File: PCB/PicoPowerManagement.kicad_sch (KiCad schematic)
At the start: 25 parts, among them J1 Conn_02x07_Odd_Even, J10 Conn_02x07_Odd_Even, J11 NAS Fan 1, J12 NAS Fan 2, J13 ATX 24P Connection, J15 Conn_01x02, J2 Conn_02x07_Odd_Even, J3 UART Header, J4 DEBUG, J5 SwitchLEDS, J6 Conn_02x07_Odd_Even, J7 Conn_02x07_Odd_Even, J8 PowerSwitch, J9 Conn_02x07_Odd_Even, Q1 2N3904, SW1 SW_SPST, U2 LP5810ADSDR, U3 LP5810ADSDR, U4 LSF0101DRYR, U5 LSF0101DRYR

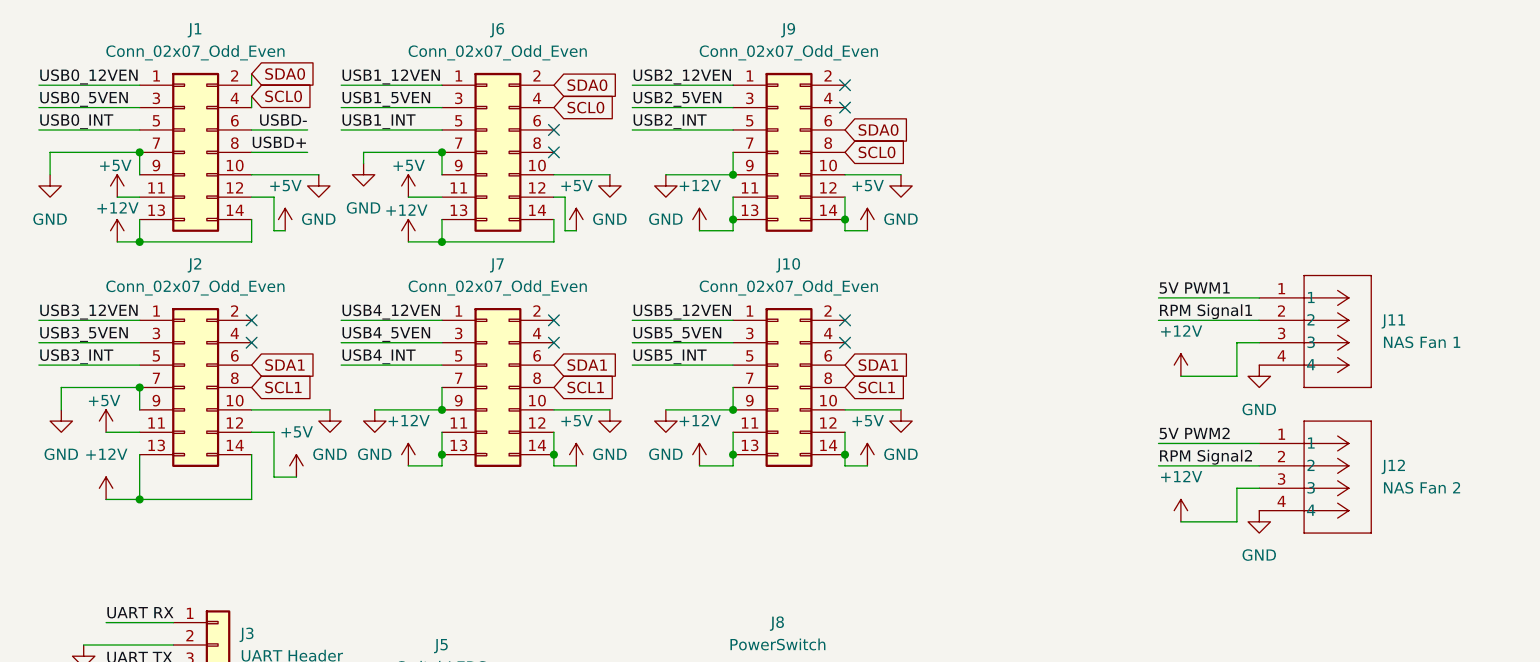
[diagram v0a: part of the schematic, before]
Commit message: confused now
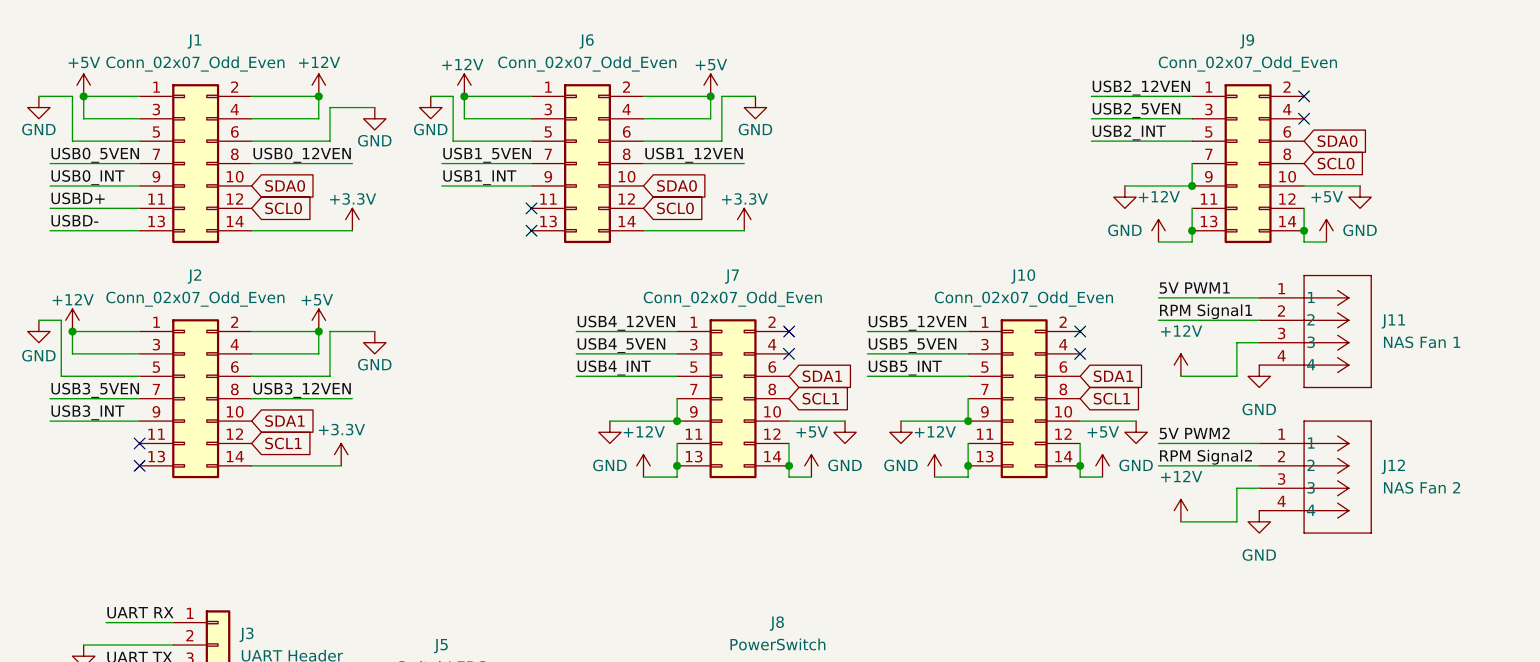
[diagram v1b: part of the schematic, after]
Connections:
- net +12V: now also J1.2 (Pin_2), J1.4 (Pin_4), J2.1 (Pin_1), J2.3 (Pin_3), J6.1 (Pin_1), J6.3 (Pin_3); no longer J1.13 (Pin_13), J1.14 (Pin_14), J2.13 (Pin_13), J2.14 (Pin_14), J6.13 (Pin_13), J6.14 (Pin_14)
- net +3.3V: now also J1.14 (Pin_14), J2.14 (Pin_14), J6.14 (Pin_14)
- net +5V: now also J1.1 (Pin_1), J1.3 (Pin_3), J2.2 (Pin_2), J2.4 (Pin_4), J6.2 (Pin_2), J6.4 (Pin_4); no longer J1.11 (Pin_11), J1.12 (Pin_12), J2.11 (Pin_11), J2.12 (Pin_12), J6.11 (Pin_11), J6.12 (Pin_12)
- net GND: now also J1.5 (Pin_5), J1.6 (Pin_6), J2.5 (Pin_5), J2.6 (Pin_6), J6.5 (Pin_5), J6.6 (Pin_6); no longer J1.10 (Pin_10), J1.7 (Pin_7), J1.9 (Pin_9), J2.10 (Pin_10), J2.7 (Pin_7), J2.9 (Pin_9), J6.10 (Pin_10), J6.7 (Pin_7), J6.9 (Pin_9)
- net SCL0: now also J1.12 (Pin_12), J6.12 (Pin_12); no longer J1.4 (Pin_4), J6.4 (Pin_4)
- net SCL1: now also J2.12 (Pin_12); no longer J2.8 (Pin_8)
- net SDA0: now also J1.10 (Pin_10), J6.10 (Pin_10); no longer J1.2 (Pin_2), J6.2 (Pin_2)
- net SDA1: now also J2.10 (Pin_10); no longer J2.6 (Pin_6)
- net USB0_12VEN: now also J1.8 (Pin_8); no longer J1.1 (Pin_1)
- net USB0_5VEN: now also J1.7 (Pin_7); no longer J1.3 (Pin_3)
- net USB0_INT: now also J1.9 (Pin_9); no longer J1.5 (Pin_5)
- net USB1_12VEN: now also J6.8 (Pin_8); no longer J6.1 (Pin_1)
- net USB1_5VEN: now also J6.7 (Pin_7); no longer J6.3 (Pin_3)
- net USB1_INT: now also J6.9 (Pin_9); no longer J6.5 (Pin_5)
- net USB3_12VEN: now also J2.8 (Pin_8); no longer J2.1 (Pin_1)
- net USB3_5VEN: now also J2.7 (Pin_7); no longer J2.3 (Pin_3)
- net USB3_INT: now also J2.9 (Pin_9); no longer J2.5 (Pin_5)
- net USBD+: now also J1.11 (Pin_11); no longer J1.8 (Pin_8)
- net USBD-: now also J1.13 (Pin_13); no longer J1.6 (Pin_6)
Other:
- moved on the sheet: J1, J10, J2, J6, J7, J9
